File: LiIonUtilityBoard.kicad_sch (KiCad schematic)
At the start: 42 parts, among them J1 USBC_Swapped, J2 Conn_02x07_Odd_Even, Q1 PMDPB30XN, U1 MAX77757JEFG420+, U2 bq298215, U3 MAX17260SETD, U4 ISL91127IR

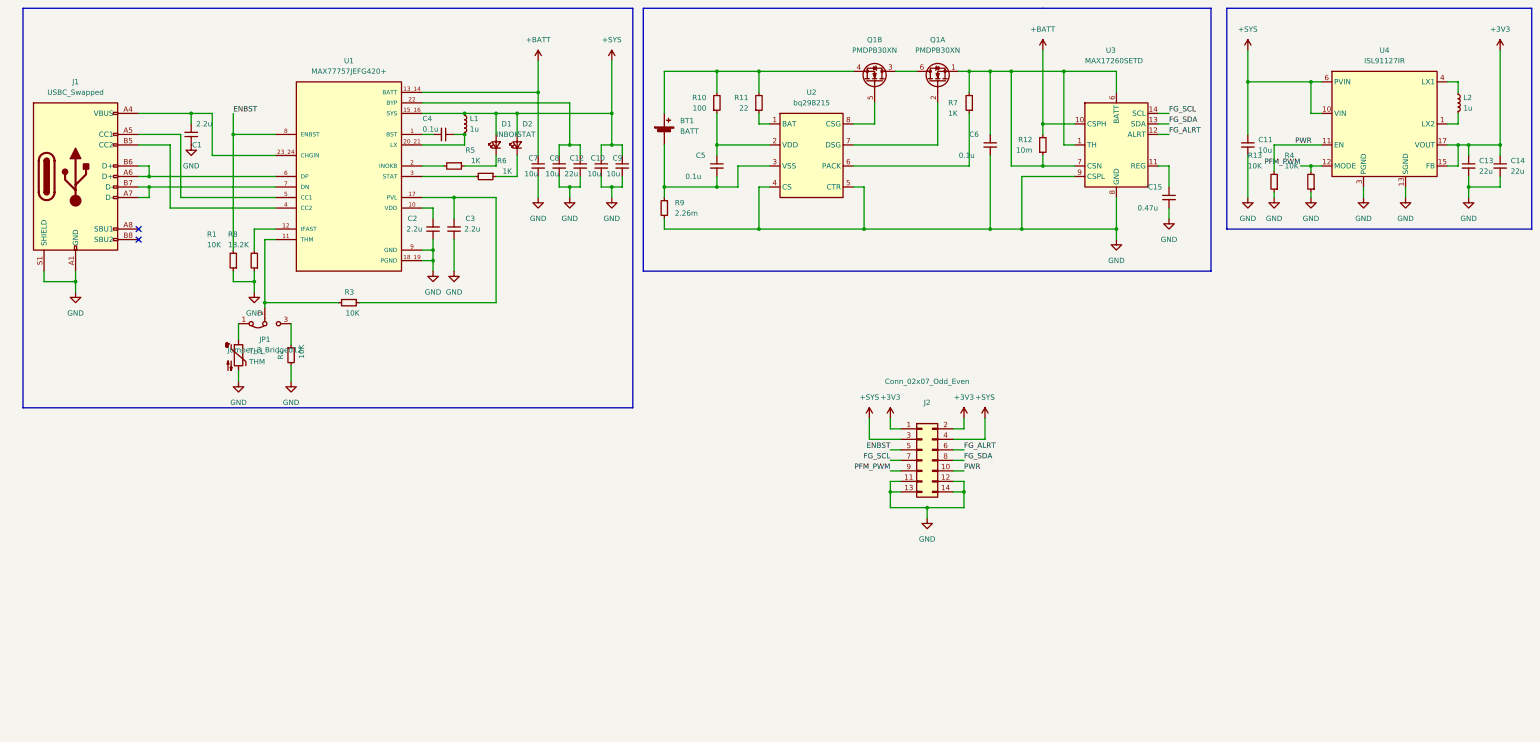
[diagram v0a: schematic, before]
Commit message: Finalize Schematic
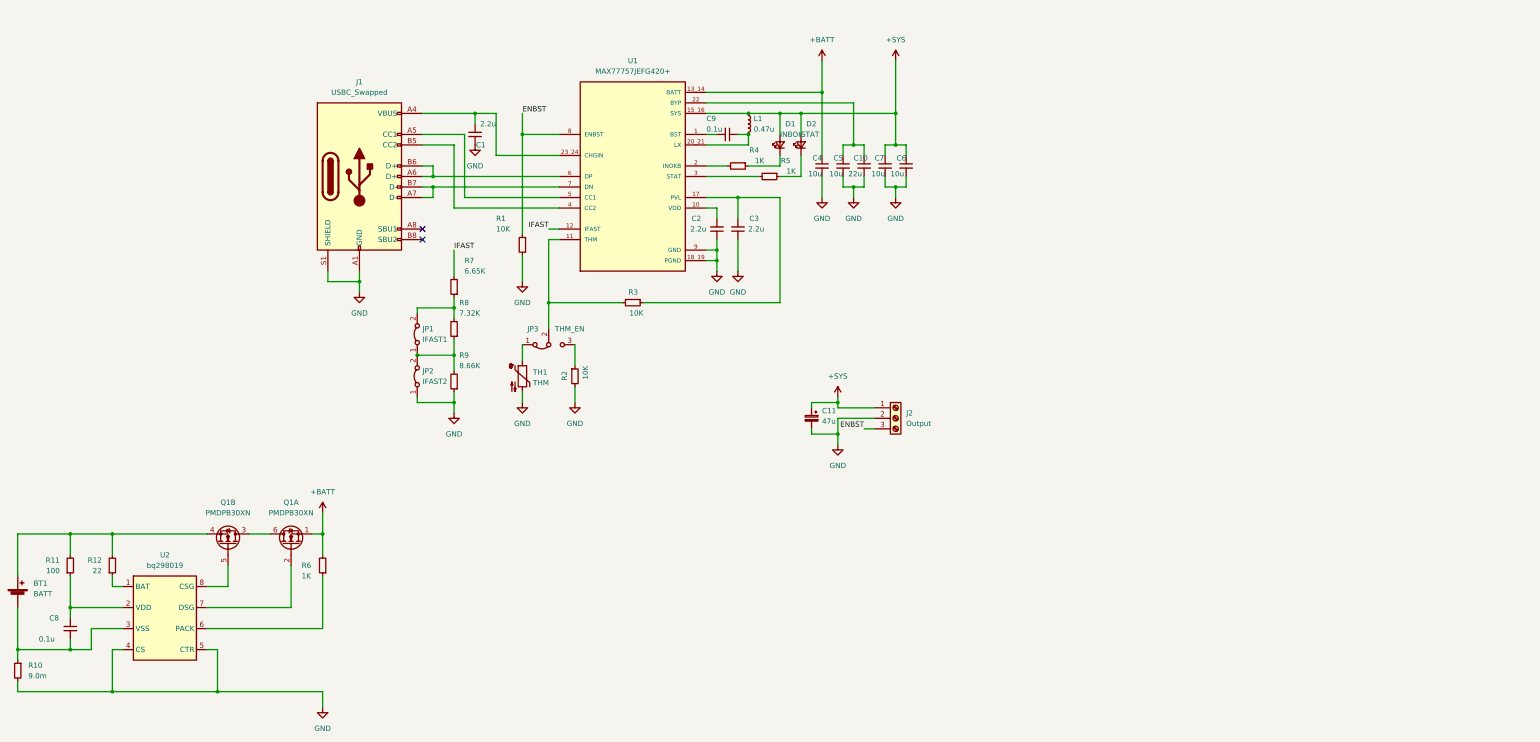
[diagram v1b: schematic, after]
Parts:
- removed C11: 10u, Capacitor_SMD:C_0805_2012Metric, symbol Device:C_Small
- removed C13, C14: 22u, Capacitor_SMD:C_0805_2012Metric, symbol Device:C_Small
- removed C15: 0.47u, Capacitor_SMD:C_0402_1005Metric, symbol Device:C_Small
- removed C6: 0.1u, Capacitor_SMD:C_0402_1005Metric, symbol Device:C_Small
- removed J2: Conn_02x07_Odd_Even, Connector_PinHeader_2.54mm:PinHeader_2x07_P2.54mm_Vertical, symbol Connector_Generic:Conn_02x07_Odd_Even
- removed L2: 1u, Inductor_SMD:L_Taiyo-Yuden_NR-60xx, symbol Device:L_Small
- removed R12: 10m, Resistor_SMD:R_0612_1632Metric, symbol Device:R_Small
- removed R13, R4: 10K, Resistor_SMD:R_0402_1005Metric, symbol Device:R_Small
- removed U2: bq298215, LUBParts:BQ298009RUGR, symbol HABParts:bq298215
- removed U3: MAX17260SETD, Package_DFN_QFN:TDFN-14-1EP_3x3mm_P0.4mm_EP1.78x2.35mm, symbol HABParts:MAX17260SETD
- removed U4: ISL91127IR, Package_DFN_QFN:QFN-20-1EP_4x4mm_P0.5mm_EP2.7x2.7mm_ThermalVias, symbol HABParts:ISL91127IR
- added C11: 47u, symbol Device:C_Polarized_Small
- added J2: Output, symbol Connector:Screw_Terminal_01x03
- added JP1: IFAST1, Jumper:SolderJumper-2_P1.3mm_Bridged_Pad1.0x1.5mm, symbol Jumper:Jumper_2_Bridged
- added JP2: IFAST2, Jumper:SolderJumper-2_P1.3mm_Bridged_Pad1.0x1.5mm, symbol Jumper:Jumper_2_Bridged
- added R8: 7.32K, symbol Device:R_Small
- added R9: 8.66K, symbol Device:R_Small
- added U2: bq298019, LUBParts:BQ298009RUGR, symbol LUBParts:bq298019
- BT1: footprint Connector_PinHeader_2.54mm:PinHeader_1x02_P2.54mm_Vertical -> (none)
- C1, C2, C3: footprint Capacitor_SMD:C_0603_1608Metric -> (none)
- C10: renamed from C12; footprint Capacitor_SMD:C_0805_2012Metric -> (none)
- C4: renamed from C7; footprint Capacitor_SMD:C_0805_2012Metric -> (none)
- C5: renamed from C8; footprint Capacitor_SMD:C_0805_2012Metric -> (none)
- C6: renamed from C9; footprint Capacitor_SMD:C_0805_2012Metric -> (none)
- C7: renamed from C10; footprint Capacitor_SMD:C_0805_2012Metric -> (none)
- C8: renamed from C5; footprint Capacitor_SMD:C_0402_1005Metric -> (none)
- C9: renamed from C4; footprint Capacitor_SMD:C_0402_1005Metric -> (none)
- JP3: renamed from JP1; value Jumper_3_Bridged12 -> THM_EN
- L1: value 1u -> 0.47u; footprint Inductor_SMD:L_Taiyo-Yuden_NR-60xx -> (none)
- Q1: footprint LUBParts:DMN1025UFDB7 -> LUBParts:SON65P200X200X65-8N
- R1, R2, R3: footprint Resistor_SMD:R_0402_1005Metric -> (none)
- R10: renamed from R9; value 2.26m -> 9.0m; footprint Resistor_SMD:R_2512_6332Metric -> (none)
- R11: renamed from R10; footprint Resistor_SMD:R_0402_1005Metric -> (none)
- R12: renamed from R11; footprint Resistor_SMD:R_0402_1005Metric -> (none)
- R4: renamed from R5; footprint Resistor_SMD:R_0603_1608Metric -> (none)
- R5: renamed from R6; footprint Resistor_SMD:R_0603_1608Metric -> (none)
- R6: renamed from R7; footprint Resistor_SMD:R_0603_1608Metric -> (none)
- R7: renamed from R8; value 18.2K -> 6.65K; footprint Resistor_SMD:R_0402_1005Metric -> (none)
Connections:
- net +BATT: now also Q1.1 (S1), R6.2
- net +SYS: now also C11.1, J2.1 (Pin_1)
- net ENBST: now also J2.3 (Pin_3)
- net GND: now also C11.2, J2.2 (Pin_2), JP2.1 (A), R9.1, U2.4 (CS), U2.5 (CTR); no longer R7.1
- net at C8.1, R11.1: now also U2.2 (VDD)
- net at BT1.2 (-), C8.2, R10.1: now also U2.3 (VSS)
- net IFAST: now reaches R7.2, U1.12 (IFAST)
- net at Q1.5 (G2): now also U2.8 (CSG)
- net at Q1.2 (G1): now also U2.7 (DSG)
- net at R12.1: now also U2.1 (BAT)
- net at R6.1: now also U2.6 (PACK)
- new net: JP1.2 (B), R7.1, R8.2
- new net: JP1.1 (A), JP2.2 (B), R8.1, R9.2
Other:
- moved on the sheet: BT1, C1, C10, C2, C3, C4, C5, C6, C7, C8, C9, D1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
